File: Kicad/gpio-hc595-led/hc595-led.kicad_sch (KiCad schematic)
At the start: 23 parts, among them K1 GPIO IN, K2 GPIO OUT, U1 74HC595, U2 3M-SJ5376

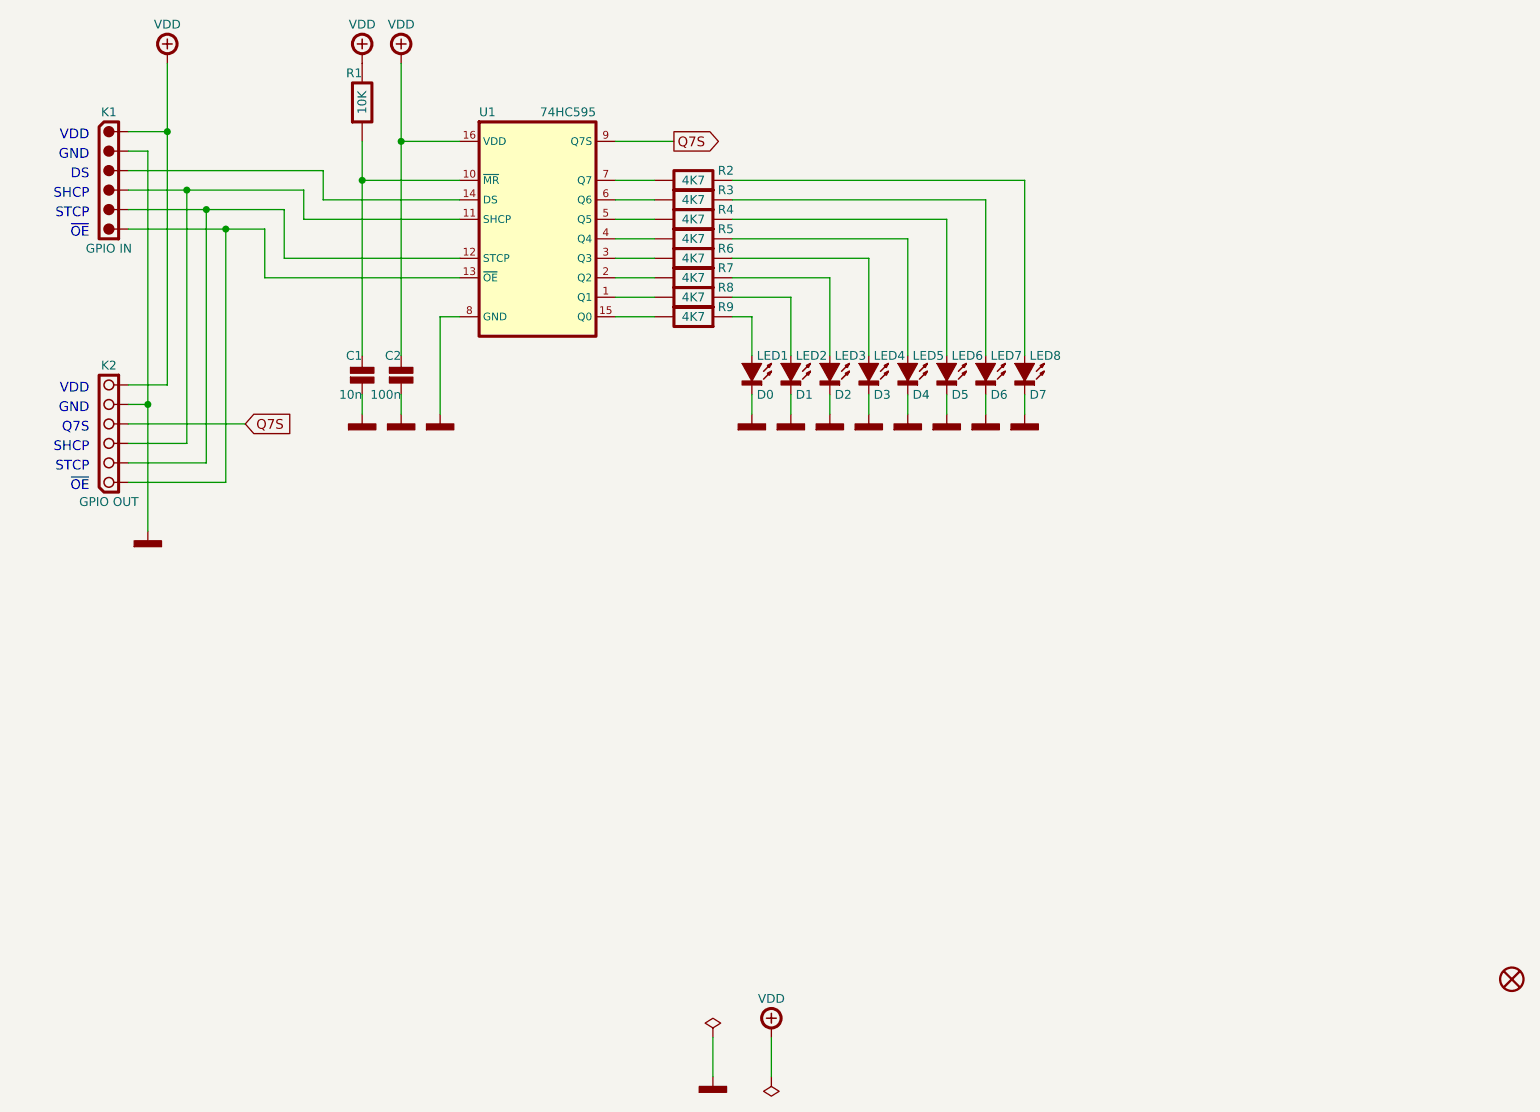
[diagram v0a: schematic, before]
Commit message: Update
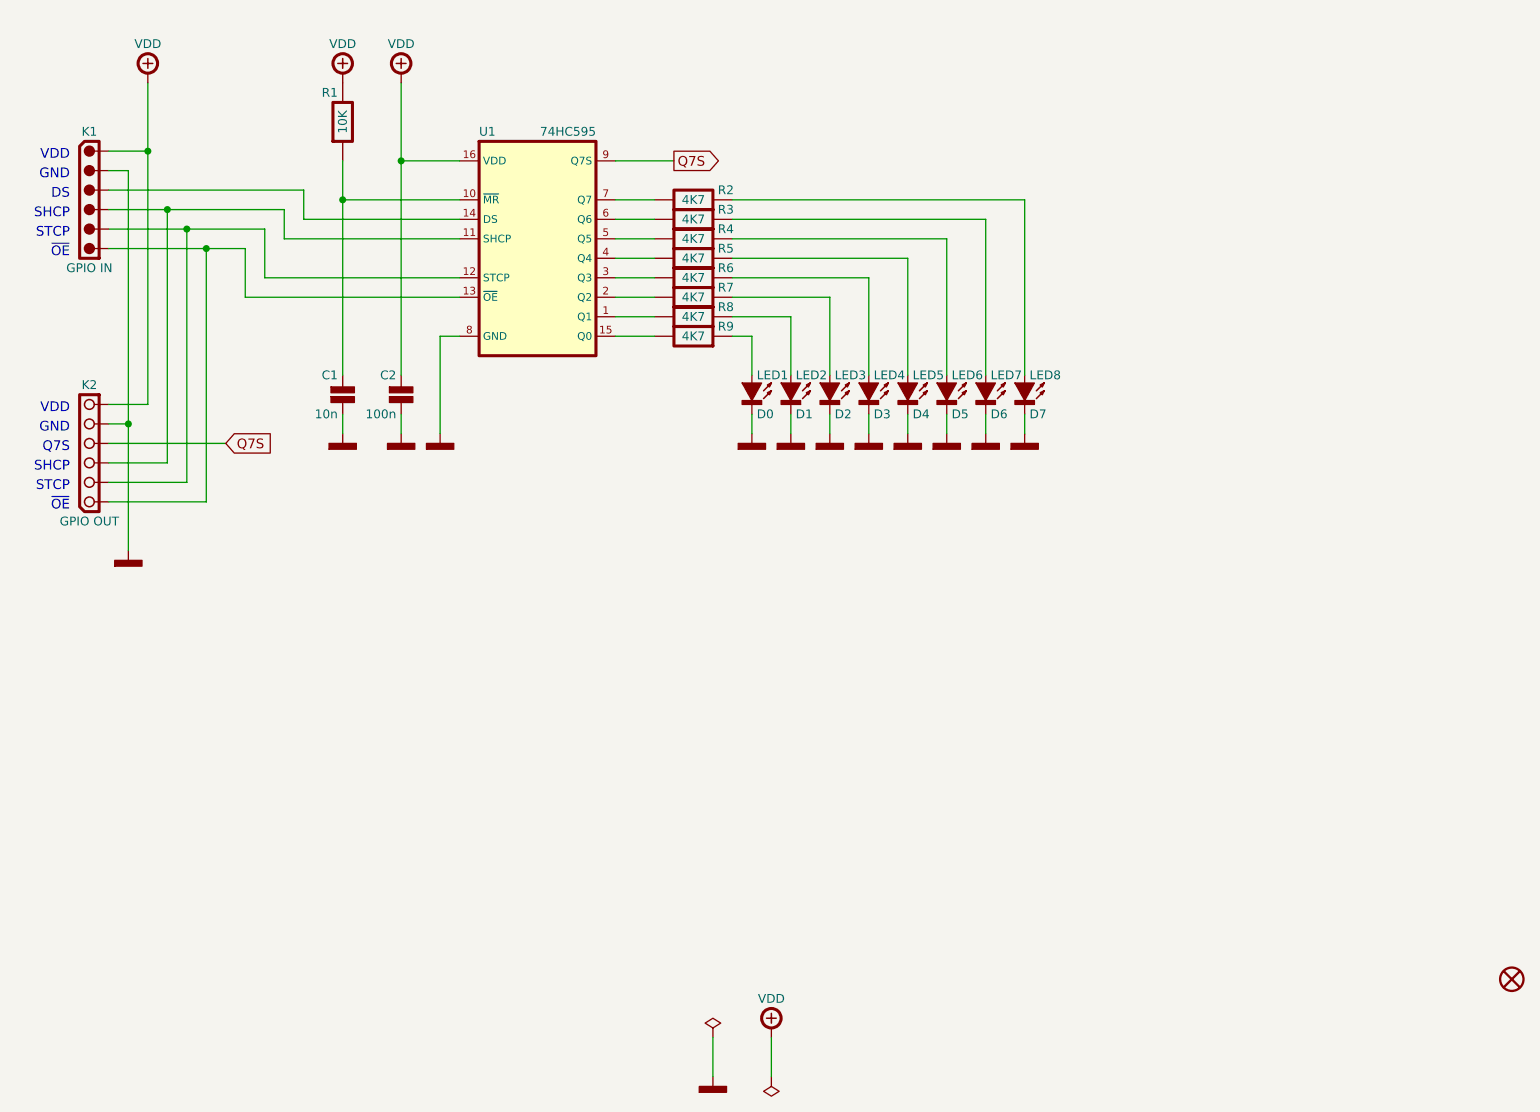
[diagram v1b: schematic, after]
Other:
- moved on the sheet: C1, C2, K1, K2, LED1, LED2, LED3, LED4, LED5, LED6, LED7, LED8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

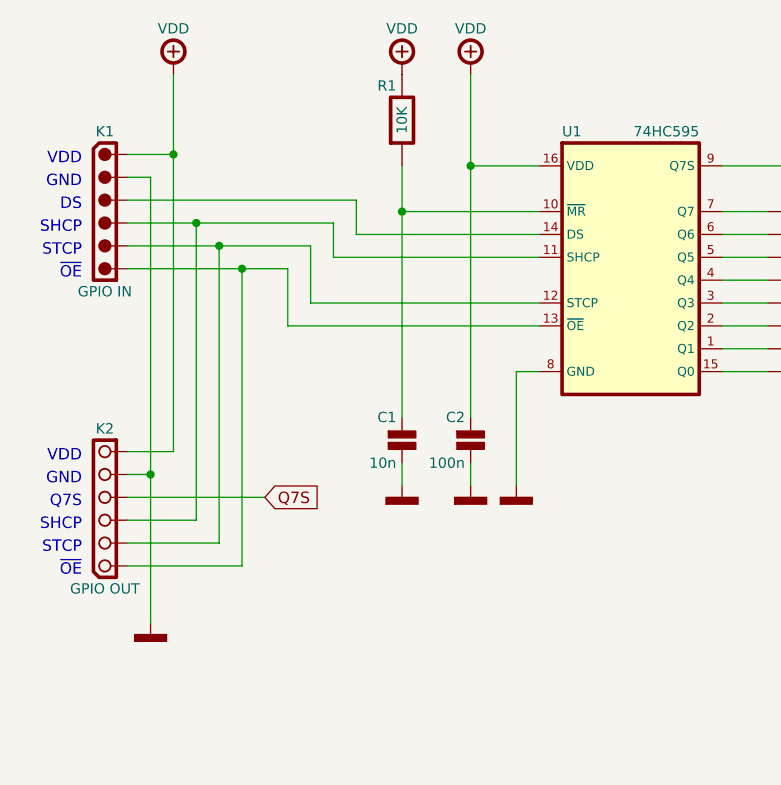
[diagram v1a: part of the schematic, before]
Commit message: Update
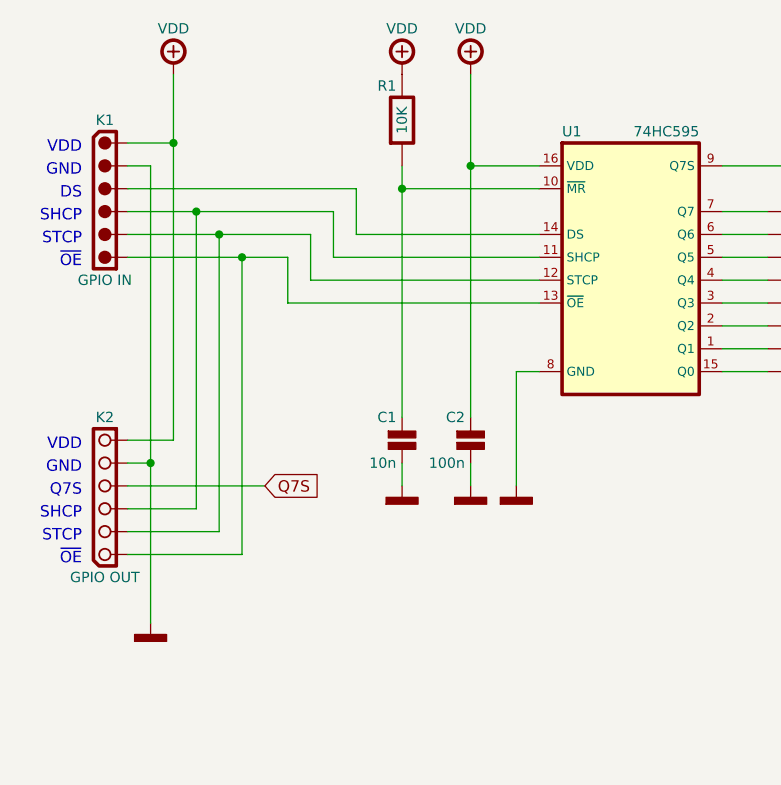
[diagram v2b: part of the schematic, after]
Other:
- moved on the sheet: K1, K2
